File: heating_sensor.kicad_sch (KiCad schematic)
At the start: 3 parts

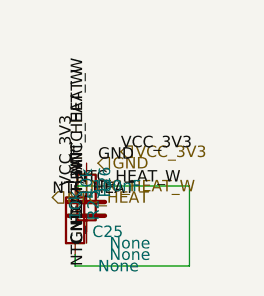
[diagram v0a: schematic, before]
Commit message: fic placer for small schemes
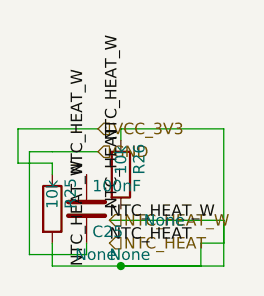
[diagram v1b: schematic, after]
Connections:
- net NTC_HEAT_W: no longer R25.1
- new net VCC_3V3: R25.1
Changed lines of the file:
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@@
 		(instances
 			(project "Untitled"
-				(path "/877ebbf2-9da6-4fab-8a1c-67fe445f8f21"
+				(path "/2b46367b-7f7a-4d0b-a981-14ef6f17f746"
 					(reference "C25")
 					(unit 1)
@@
 	(symbol
 		(lib_id "Device:R")
-		(at 16.51 19.05 0)
+		(at 13.97 17.78 0)
 		(unit 1)
 		(exclude_from_sim no)
@@
 		(fields_autoplaced no)
 		(property "Reference" "R25"
-			(at 18.542 19.05 90)
+			(at 16.002 17.78 90)
 			(effects
 				(font
@@
 		)
 		(property "Value" "10k"
-			(at 16.51 19.05 90)
+			(at 13.97 17.78 90)
 			(effects
 				(font
@@
 		)
 		(property "mirror" "None"
-			(at 19.05 24.1299 0)
+			(at 16.51 22.8599 0)
 			(effects
 				(font
@@
 		(instances
 			(project "Untitled"
-				(path "/877ebbf2-9da6-4fab-8a1c-67fe445f8f21"
+				(path "/2b46367b-7f7a-4d0b-a981-14ef6f17f746"
 					(reference "R25")
 					(unit 1)
@@
 	(symbol
 		(lib_id "Device:R")
-		(at 17.78 16.51 0)
+		(at 21.59 13.97 0)
 		(unit 1)
 		(exclude_from_sim no)
@@
 		(fields_autoplaced no)
 		(property "Reference" "R26"
-			(at 19.812 16.51 90)
+			(at 23.622 13.97 90)
 			(effects
 				(font
@@
 		)
 		(property "Value" "10k"
-			(at 17.78 16.51 90)
+			(at 21.59 13.97 90)
 			(effects
 				(font
@@
 		)
 		(property "mirror" "None"
-			(at 20.32 21.5899 0)
+			(at 24.13 19.0499 0)
 			(effects
 				(font
@@
 		(instances
 			(project "Untitled"
-				(path "/877ebbf2-9da6-4fab-8a1c-67fe445f8f21"
+				(path "/2b46367b-7f7a-4d0b-a981-14ef6f17f746"
 					(reference "R26")
 					(unit 1)
@@
 	(wire
 		(pts
-			(xy 16.51 22.86) (xy 16.51 24.13)
-		)
-		(stroke
-			(width 0)
-			(type default)
-		)
-	)
-	(wire
-		(pts
-			(xy 16.51 24.13) (xy 29.21 24.13)
-		)
-		(stroke
-			(width 0)
-			(type default)
-		)
-	)
-	(wire
-		(pts
-			(xy 29.21 24.13) (xy 29.21 15.24)
-		)
-		(stroke
-			(width 0)
-			(type default)
-		)
-	)
-	(wire
-		(pts
-			(xy 29.21 15.24) (xy 16.51 15.24)
-		)
-		(stroke
-			(width 0)
-			(type default)
-		)
-	)
-	(label "VCC_3V3"
-		(at 16.51 15.24 90)
-		(effects
-			(font
-				(size 1.27 1.27)
-			)
-			(justify left bottom)
-		)
-	)
-	(label "VCC_3V3"
-		(at 21.59 11.43 180)
-		(effects
-			(font
-				(size 1.27 1.27)
-			)
-			(justify left bottom)
-		)
-	)
-	(label "GND"
-		(at 17.78 21.59 270)
-		(effects
-			(font
-				(size 1.27 1.27)
-			)
-			(justify left bottom)
-		)
-	)
-	(label "GND"
-		(at 19.05 12.7 180)
-		(effects
-			(font
-				(size 1.27 1.27)
-			)
-			(justify left bottom)
-		)
+			(xy 13.97 13.97) (xy 13.97 12.7)
+		)
+		(stroke
+			(width 0)
+			(type default)
+		)
+	)
+	(wire
+		(pts
+			(xy 13.97 12.7) (xy 10.16 12.7)
+		)
+		(stroke
+			(width 0)
+			(type default)
+		)
+	)
+	(wire
+		(pts
+			(xy 10.16 12.7) (xy 10.16 8.89)
+		)
+		(stroke
+			(width 0)
+			(type default)
+		)
+	)
+	(wire
+		(pts
+			(xy 10.16 8.89) (xy 19.05 8.89)
+		)
+		(stroke
+			(width 0)
+			(type default)
+		)
+	)
+	(wire
+		(pts
+			(xy 17.78 21.59) (xy 17.78 22.86)
+		)
+		(stroke
+			(width 0)
+			(type default)
+		)
+	)
+	(wire
+		(pts
+			(xy 17.78 22.86) (xy 11.43 22.86)
+		)
+		(stroke
+			(width 0)
+			(type default)
+		)
+	)
+	(wire
+		(pts
+			(xy 11.43 22.86) (xy 11.43 11.43)
+		)
+		(stroke
+			(width 0)
+			(type default)
+		)
+	)
+	(wire
+		(pts
+			(xy 11.43 11.43) (xy 13.97 11.43)
+		)
+		(stroke
+			(width 0)
+			(type default)
+		)
+	)
+	(wire
+		(pts
+			(xy 13.97 11.43) (xy 19.05 11.43)
+		)
+		(stroke
+			(width 0)
+			(type default)
+		)
+	)
+	(wire
+		(pts
+			(xy 13.97 21.59) (xy 13.97 24.13)
+		)
+		(stroke
+			(width 0)
+			(type default)
+		)
+	)
+	(wire
+		(pts
+			(xy 13.97 24.13) (xy 33.02 24.13)
+		)
+		(stroke
+			(width 0)
+			(type default)
+		)
+	)
+	(wire
+		(pts
+			(xy 33.02 24.13) (xy 33.02 19.05)
+		)
+		(stroke
+			(width 0)
+			(type default)
+		)
+	)
+	(wire
+		(pts
+			(xy 33.02 19.05) (xy 20.32 19.05)
+		)
+		(stroke
+			(width 0)
+			(type default)
+		)
+	)
+	(wire
+		(pts
+			(xy 21.59 10.16) (xy 21.59 8.89)
+		)
+		(stroke
+			(width 0)
+			(type default)
+		)
+	)
+	(wire
+		(pts
+			(xy 21.59 8.89) (xy 33.02 8.89)
+		)
+		(stroke
+			(width 0)
+			(type default)
+		)
+	)
+	(wire
+		(pts
+			(xy 33.02 8.89) (xy 33.02 21.59)
+		)
+		(stroke
+			(width 0)
+			(type default)
+		)
+	)
+	(wire
+		(pts
+			(xy 33.02 21.59) (xy 30.48 21.59)
+		)
+		(stroke
+			(width 0)
+			(type default)
+		)
+	)
+	(wire
+		(pts
+			(xy 30.48 21.59) (xy 30.48 24.13)
+		)
+		(stroke
+			(width 0)
+			(type default)
+		)
+	)
+	(wire
+		(pts
+			(xy 30.48 24.13) (xy 21.59 24.13)
+		)
+		(stroke
+			(width 0)
+			(type default)
+		)
+	)
+	(junction
+		(at 21.59 24.13)
+		(diameter 0)
+		(color 0 0 0 0)
 	)
 	(label "NTC_HEAT_W"
@@
 	)
 	(label "NTC_HEAT_W"
-		(at 17.78 12.7 90)
+		(at 21.59 10.16 90)
 		(effects
 			(font
@@
 	)
 	(label "NTC_HEAT_W"
-		(at 16.51 15.24 0.0000)
+		(at 20.32 19.05 0.0000)
 		(effects
 			(font
@@
 	)
 	(label "NTC_HEAT"
-		(at 17.78 20.32 270)
+		(at 21.59 17.78 270)
 		(effects
 			(font
@@
 	)
 	(label "NTC_HEAT"
-		(at 13.97 16.51 0.0000)
+		(at 20.32 21.59 0.0000)
 		(effects
 			(font
@@
 	(hierarchical_label "VCC_3V3"
 		(shape input)
-		(at 21.59 11.43 180)
+		(at 19.05 8.89 180)
 		(effects
 			(font
@@
 	(hierarchical_label "GND"
 		(shape input)
-		(at 19.05 12.7 180)
+		(at 19.05 11.43 180)
 		(effects
 			(font
@@
 	(hierarchical_label "NTC_HEAT_W"
 		(shape input)
-		(at 16.51 15.24 0)
+		(at 20.32 19.05 0)
 		(effects
 			(font
@@
 	(hierarchical_label "NTC_HEAT"
 		(shape input)
-		(at 13.97 16.51 0)
-		(effects
-			(font
+		(at 20.32 21.59 0)
+		(effects
+			(font
